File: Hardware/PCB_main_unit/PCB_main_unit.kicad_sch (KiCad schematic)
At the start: 46 parts, among them J1 Conn_01x03, J10 Conn_01x03, J11 Conn_01x03, J12 Conn_01x04, J13 Conn_01x07, J14 Conn_ST_STDC14, J15 Conn_01x03, J2 Conn_01x03, J3 Conn_01x03, J4 Conn_01x03, J5 Conn_01x03, J6 Conn_01x03, J7 Conn_01x03, J8 Conn_01x03, J9 Conn_01x06, U2 STM32G474RETx, U3 AZ1117-3.3

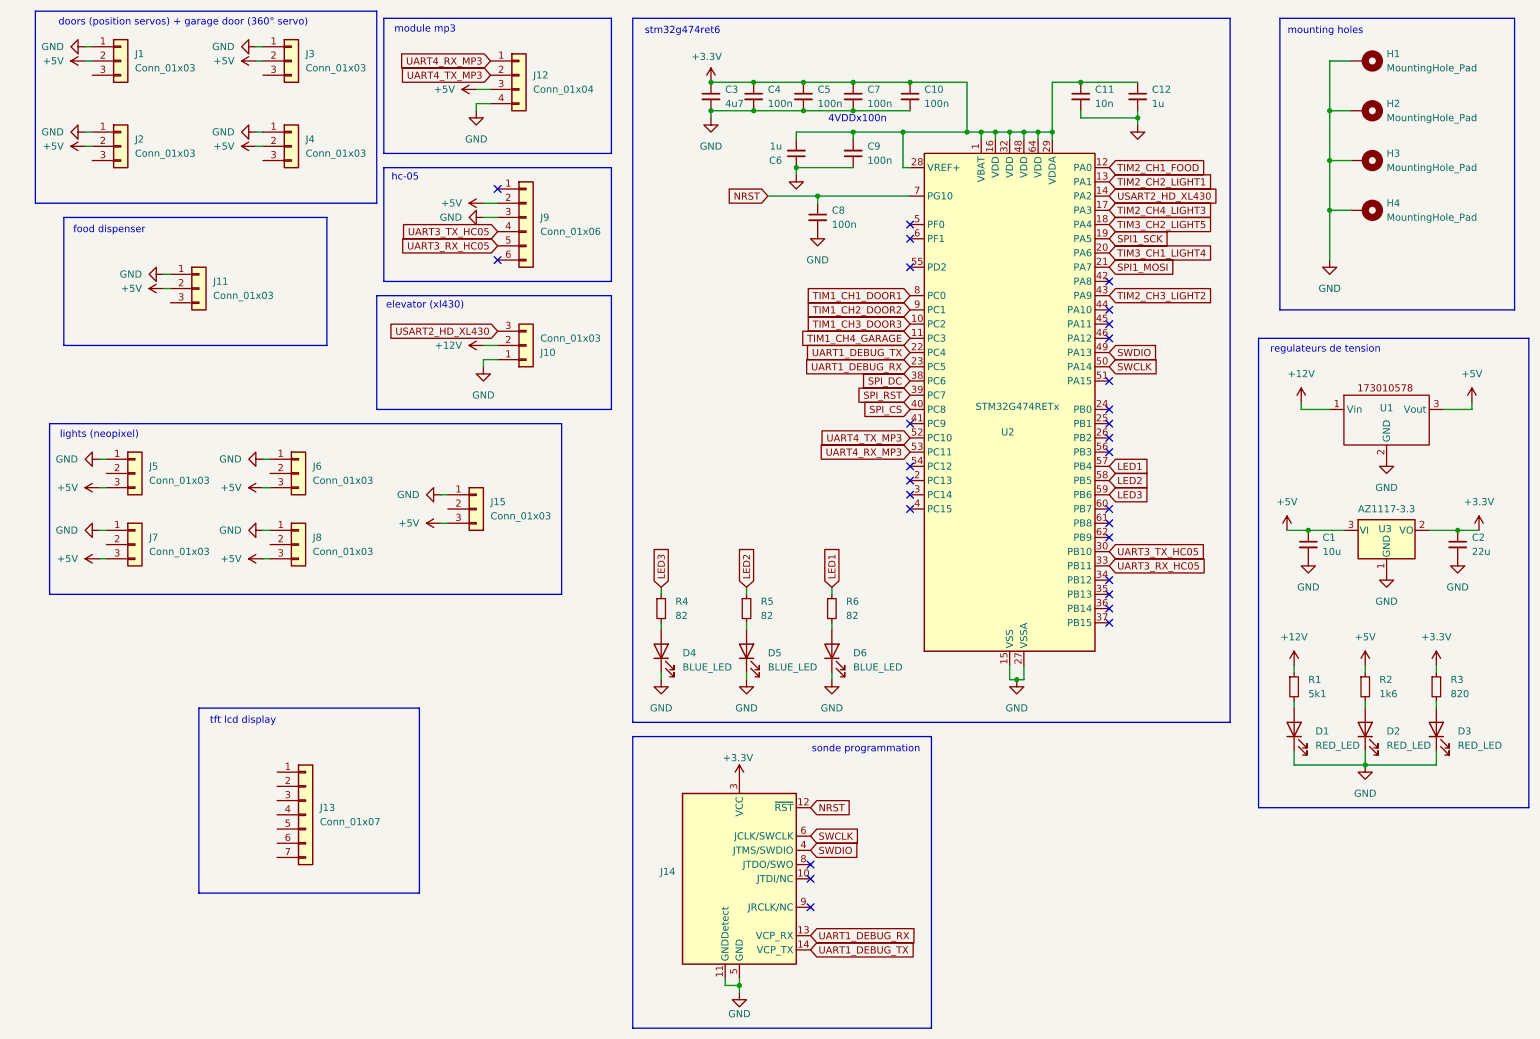
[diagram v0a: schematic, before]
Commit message: finished main unit schematic
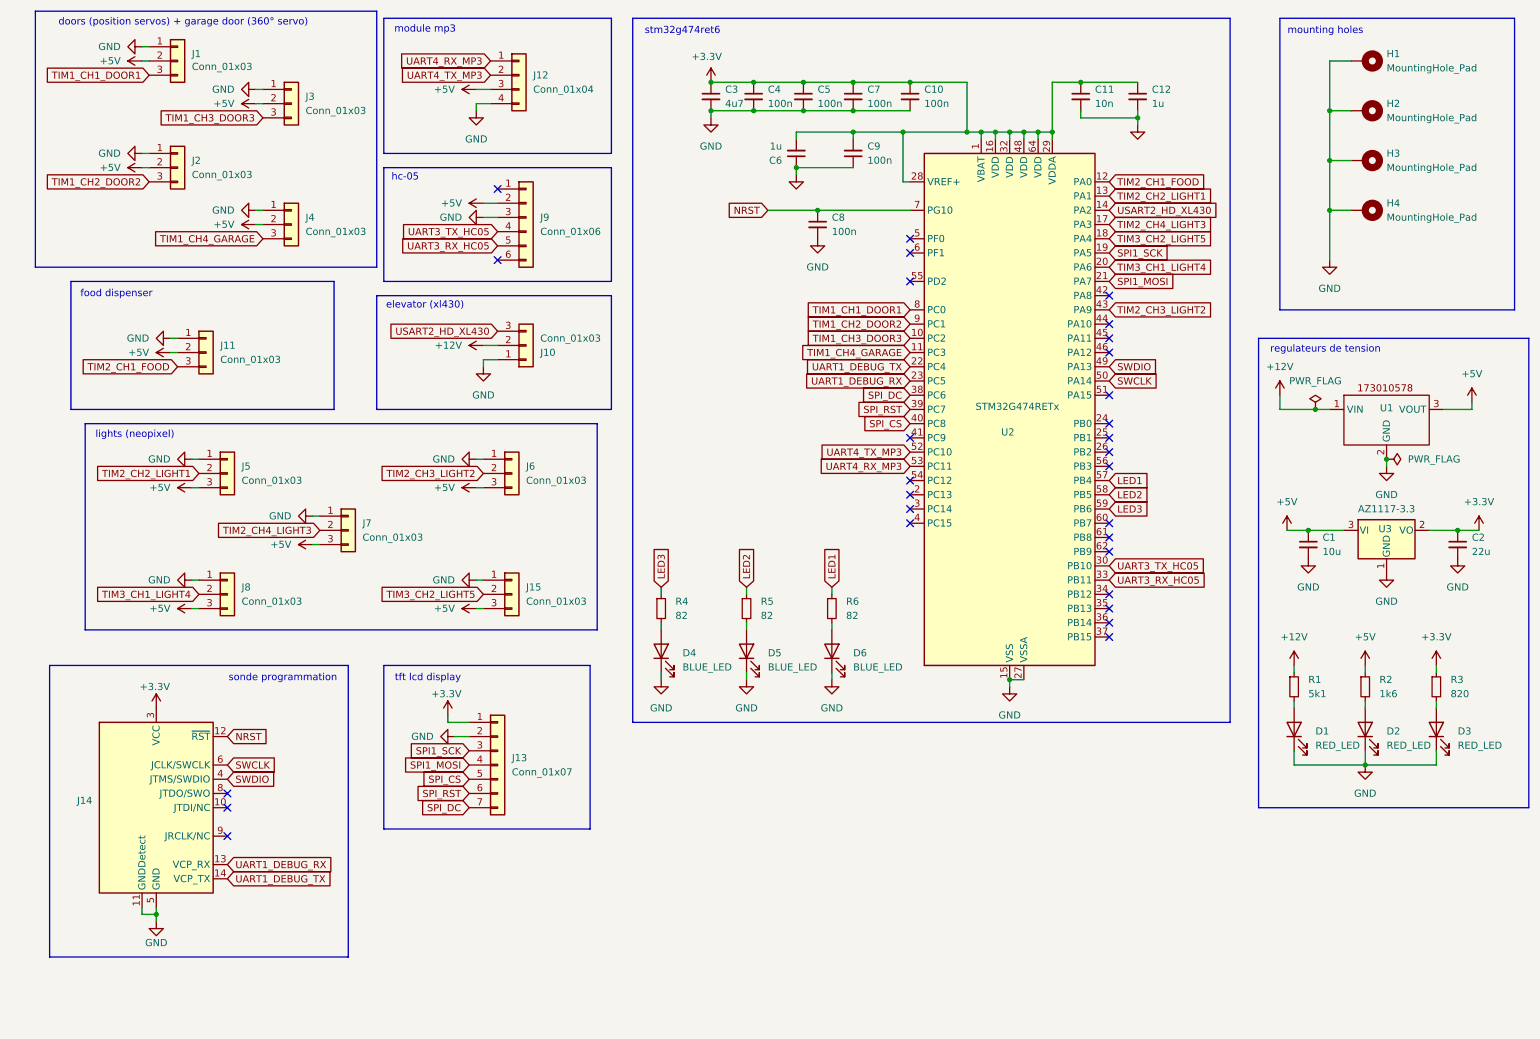
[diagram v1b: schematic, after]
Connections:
- net +3.3V: now also J13.1 (Pin_1)
- net GND: now also J13.2 (Pin_2)
- net SPI1_MOSI: now also J13.4 (Pin_4)
- net SPI1_SCK: now also J13.3 (Pin_3)
- net SPI_CS: now also J13.5 (Pin_5)
- net SPI_DC: now also J13.7 (Pin_7)
- net SPI_RST: now also J13.6 (Pin_6)
- net TIM1_CH1_DOOR1: now also J1.3 (Pin_3)
- net TIM1_CH2_DOOR2: now also J2.3 (Pin_3)
- net TIM1_CH3_DOOR3: now also J3.3 (Pin_3)
- net TIM1_CH4_GARAGE: now also J4.3 (Pin_3)
- net TIM2_CH1_FOOD: now also J11.3 (Pin_3)
- net TIM2_CH2_LIGHT1: now also J5.2 (Pin_2)
- net TIM2_CH3_LIGHT2: now also J6.2 (Pin_2)
- net TIM2_CH4_LIGHT3: now also J7.2 (Pin_2)
- net TIM3_CH1_LIGHT4: now also J8.2 (Pin_2)
- net TIM3_CH2_LIGHT5: now also J15.2 (Pin_2)
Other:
- note removed: "4VDDx100n"
- moved on the sheet: C8, J1, J11, J13, J14, J15, J2, J3, J4, J5, J6, J7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
